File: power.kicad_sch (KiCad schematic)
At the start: 14 parts, among them J1 USB_B_Micro, U2 S2B-PH-K-S-GW, U3 AP2112K-3.3TRG1, U4 MCP73831T-2ACI/OT, U6 MSK-12C02_SMD_SPDT_SWITCH

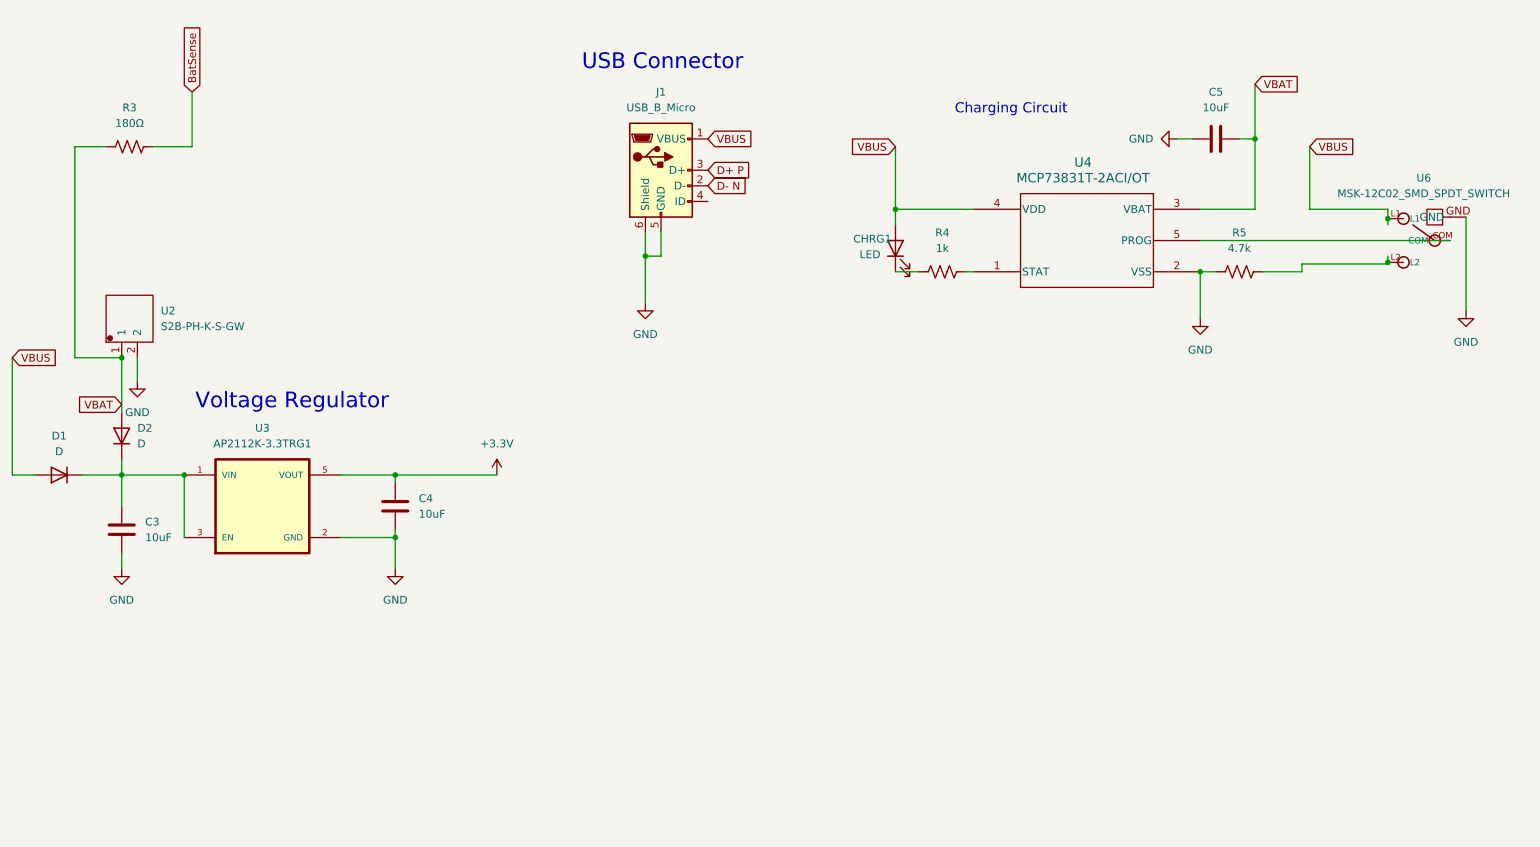
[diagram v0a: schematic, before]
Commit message: Create prelim PCB
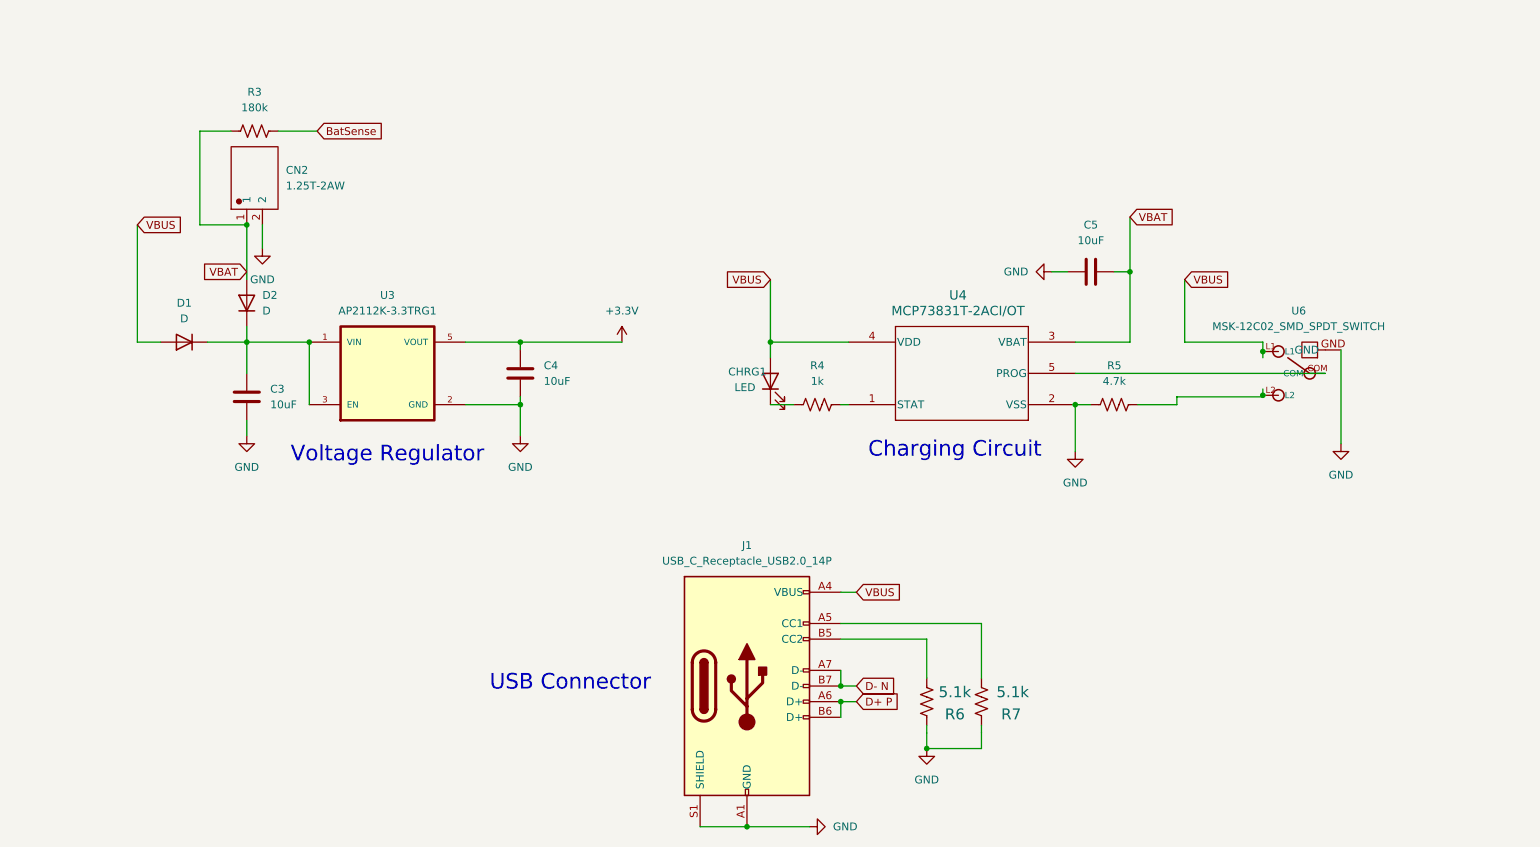
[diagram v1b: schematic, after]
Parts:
- removed J1: USB_B_Micro, Connector_USB:USB_Micro-B_Amphenol_10103594-0001LF_Horizontal, symbol uSlime:USB_B_Micro
- removed U2: S2B-PH-K-S-GW, Connector_JST:JST_PH_S2B-PH-K_1x02_P2.00mm_Horizontal, symbol uSlime:S2B-PH-K-S-GW
- added CN2: 1.25T-2AW, uSlime-libs:CONN-TH_2P-P1.25_1.25T-2AW, symbol uSlime:1.25T-2AW
- added J1: USB_C_Receptacle_USB2.0_14P, Connector_USB:USB_C_Receptacle_GCT_USB4105-xx-A_16P_TopMnt_Horizontal, symbol uSlime:USB_C_Receptacle_USB2.0_14P
- added R6, R7: 5.1k, Resistor_SMD:R_0402_1005Metric, symbol uSlime:R_US
- D1, D2: footprint Diode_SMD:D_0603_1608Metric -> Diode_SMD:D_0402_1005Metric
- R3: value 180Ω -> 180k
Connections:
- net D+ P: now also J1.A6 (D+), J1.B6 (D+)
- net D- N: now also J1.A7 (D-), J1.B7 (D-)
- net GND: now also CN2.2, J1.A1 (GND), J1.A12 (GND), J1.B1 (GND), J1.B12 (GND), J1.S1 (SHIELD), R6.1, R7.1
- net VBAT: now also CN2.1
- net VBUS: now also J1.A4 (VBUS), J1.A9 (VBUS), J1.B4 (VBUS), J1.B9 (VBUS)
- new net: J1.A5 (CC1), R7.2
- new net: J1.B5 (CC2), R6.2
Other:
- moved on the sheet: C3, C4, C5, CHRG1, D1, D2, R3, R4, R5, U3, U4, U6
